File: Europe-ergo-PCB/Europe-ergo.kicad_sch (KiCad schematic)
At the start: 230 parts, among them J1 Conn_01x04_Male/I2C, J2 Conn_01x04_Male, SW1 MX-NO-LED, SW10 MX-NO-LED, SW11 MX-NO-LED, SW12 MX-NO-LED, SW13 MX-NO-LED, SW14 MX-NO-LED, SW15 MX-NO-LED, SW16 MX-NO-LED, SW17 MX-NO-LED, SW18 MX-NO-LED, SW19 MX-NO-LED, SW2 MX-NO-LED, SW20 MX-NO-LED, SW21 MX-NO-LED, SW22 MX-NO-LED, SW23 MX-NO-LED, SW24 MX-NO-LED, SW25 MX-NO-LED, SW26 MX-NO-LED, SW27 MX-NO-LED, SW28 MX-NO-LED, SW29 MX-NO-LED, SW3 MX-NO-LED, SW30 MX-NO-LED, SW31 MX-NO-LED, SW32 MX-NO-LED, SW33 MX-NO-LED, SW34 MX-NO-LED, SW35 MX-NO-LED, SW36 MX-NO-LED, SW37 MX-NO-LED, SW38 MX-NO-LED, SW39 MX-NO-LED, SW4 MX-NO-LED, SW40 MX-NO-LED, SW41 MX-NO-LED, SW42 MX-NO-LED, SW43 MX-NO-LED, SW44 MX-NO-LED, SW45 MX-NO-LED, SW46 MX-NO-LED, SW47 MX-NO-LED, SW48 SW_Push, SW49 SW_Push, SW5 MX-NO-LED, SW50 MX-NO-LED, SW51 MX-NO-LED, SW52 MX-NO-LED, SW53 MX-NO-LED, SW54 MX-NO-LED, SW55 MX-NO-LED, SW56 MX-NO-LED, SW57 MX-NO-LED, SW58 MX-NO-LED, SW59 MX-NO-LED, SW6 MX-NO-LED, SW60 MX-NO-LED, SW61 MX-NO-LED, SW62 MX-NO-LED, SW63 MX-NO-LED, SW64 MX-NO-LED, SW65 MX-NO-LED, SW66 MX-NO-LED, SW67 MX-NO-LED, SW68 MX-NO-LED, SW69 MX-NO-LED, SW7 MX-NO-LED, SW70 MX-NO-LED, SW71 MX-NO-LED, SW72 MX-NO-LED, SW73 MX-NO-LED, SW74 MX-NO-LED, SW75 MX-NO-LED, SW76 MX-NO-LED, SW77 MX-NO-LED, SW78 MX-NO-LED, SW79 MX-NO-LED, SW8 MX-NO-LED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

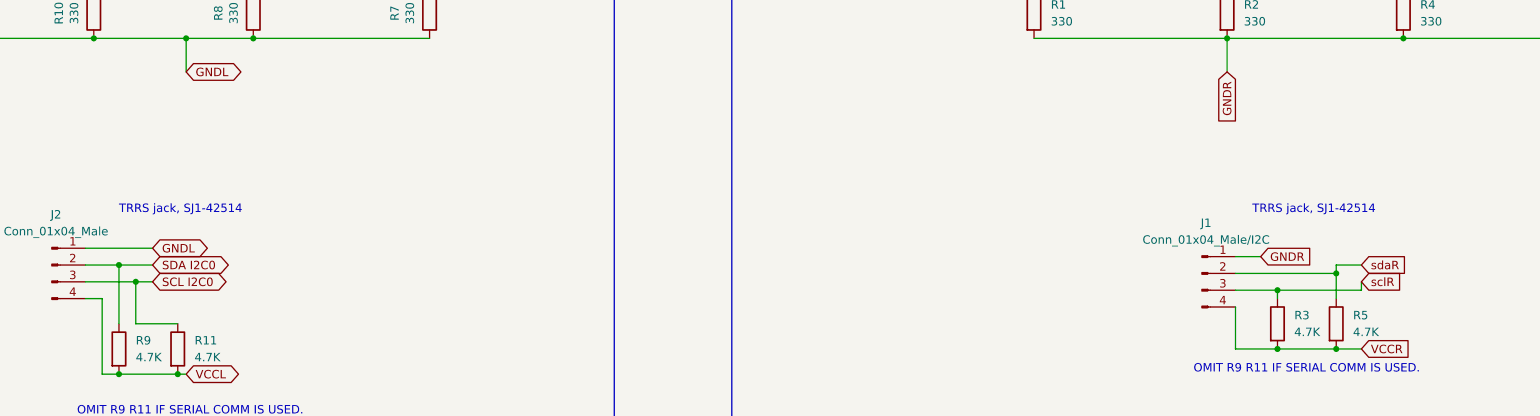
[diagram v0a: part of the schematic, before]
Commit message: Add files via upload
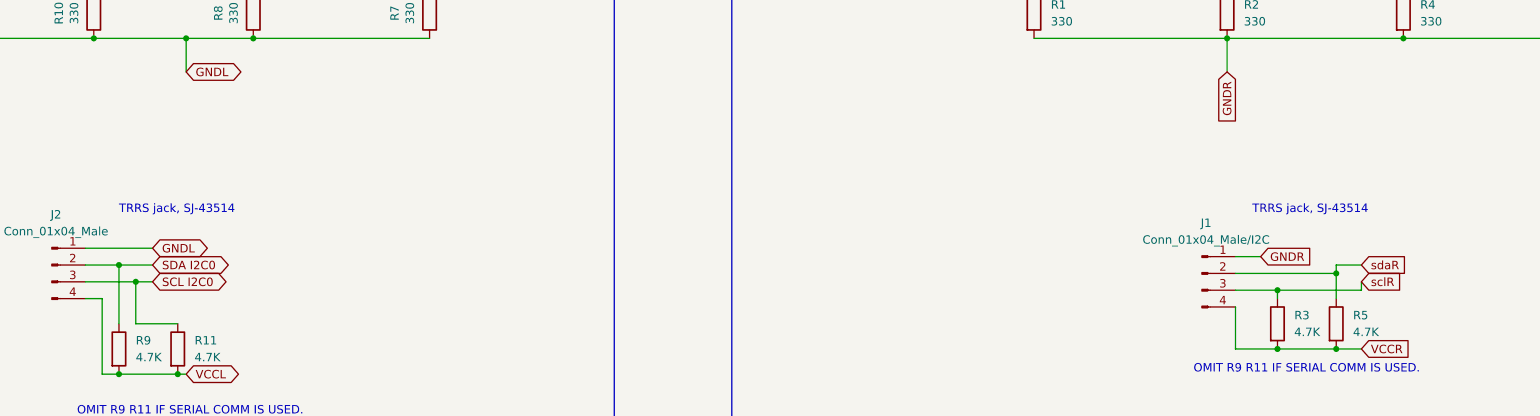
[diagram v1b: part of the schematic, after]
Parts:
- J1, J2: footprint Connector_Audio:Jack_3.5mm_CUI_SJ1-43514_Horizontal -> switch:CUI_SJ-43514
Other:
- note added: "TRRS jack, SJ-43514"
- note removed: "TRRS jack, SJ1-42514"
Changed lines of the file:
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@@
     (effects (font (size 1.27 1.27)) (justify left bottom))
   )
-  (text "TRRS jack, SJ1-42514" (at 496.57 176.53 0)
+  (text "TRRS jack, SJ-43514" (at 496.57 176.53 0)
     (effects (font (size 1.27 1.27)) (justify left bottom))
   )
@@
     (effects (font (size 1.27 1.27)) (justify left bottom))
   )
-  (text "TRRS jack, SJ1-42514" (at 325.12 176.53 0)
+  (text "TRRS jack, SJ-43514" (at 325.12 176.53 0)
     (effects (font (size 1.27 1.27)) (justify left bottom))
   )
@@
     (property "Reference" "J1" (id 0) (at 489.585 177.8 0))
     (property "Value" "Conn_01x04_Male/I2C" (id 1) (at 489.585 180.34 0))
-    (property "Footprint" "Connector_Audio:Jack_3.5mm_CUI_SJ1-43514_Horizontal" (id 2) (at 488.95 185.42 0)
+    (property "Footprint" "switch:CUI_SJ-43514" (id 2) (at 488.95 185.42 0)
       (effects (font (size 1.27 1.27)) hide)
     )
@@
     (property "Reference" "J2" (id 0) (at 315.595 176.53 0))
     (property "Value" "Conn_01x04_Male" (id 1) (at 315.595 179.07 0))
-    (property "Footprint" "Connector_Audio:Jack_3.5mm_CUI_SJ1-43514_Horizontal" (id 2) (at 314.96 184.15 0)
+    (property "Footprint" "switch:CUI_SJ-43514" (id 2) (at 314.96 184.15 0)
       (effects (font (size 1.27 1.27)) hide)
     )
@@
     )
     (path "/bcbf6456-a268-4571-98a7-f76d400f1e35"
-      (reference "J1") (unit 1) (value "Conn_01x04_Male/I2C") (footprint "Connector_Audio:Jack_3.5mm_CUI_SJ1-43514_Horizontal")
+      (reference "J1") (unit 1) (value "Conn_01x04_Male/I2C") (footprint "switch:CUI_SJ-43514")
     )
     (path "/bd999351-9dec-4c6e-be4f-9dc843edca2c"
-      (reference "J2") (unit 1) (value "Conn_01x04_Male") (footprint "Connector_Audio:Jack_3.5mm_CUI_SJ1-43514_Horizontal")
+      (reference "J2") (unit 1) (value "Conn_01x04_Male") (footprint "switch:CUI_SJ-43514")
     )
     (path "/9150a2db-2c19-4fd2-898c-5626ac1ec48b"
